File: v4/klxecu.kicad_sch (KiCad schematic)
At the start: 15 parts, among them J1 cam_sensor, J2 Conn_01x06, U1 S36B-WPZK-A, U2 LM2940S-5.0/NOPB, U3 Arduino Mega 2560 Pro

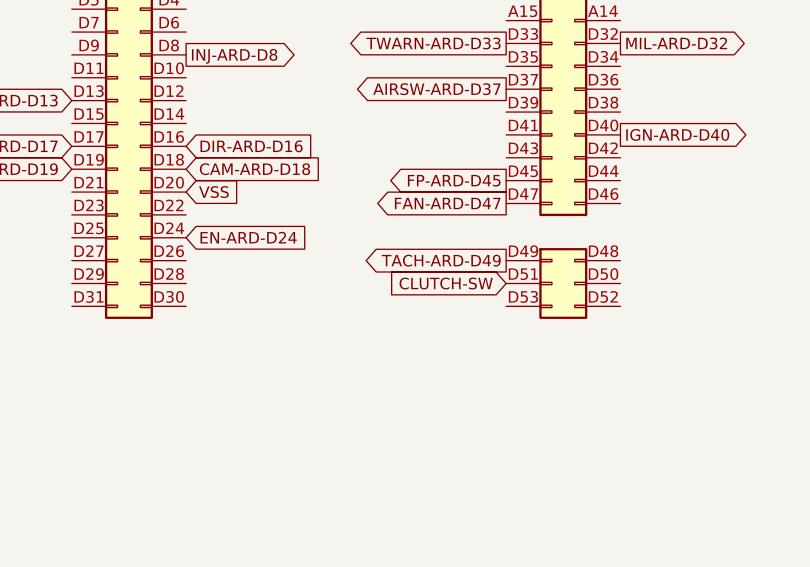
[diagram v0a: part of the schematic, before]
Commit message: V4 potential design
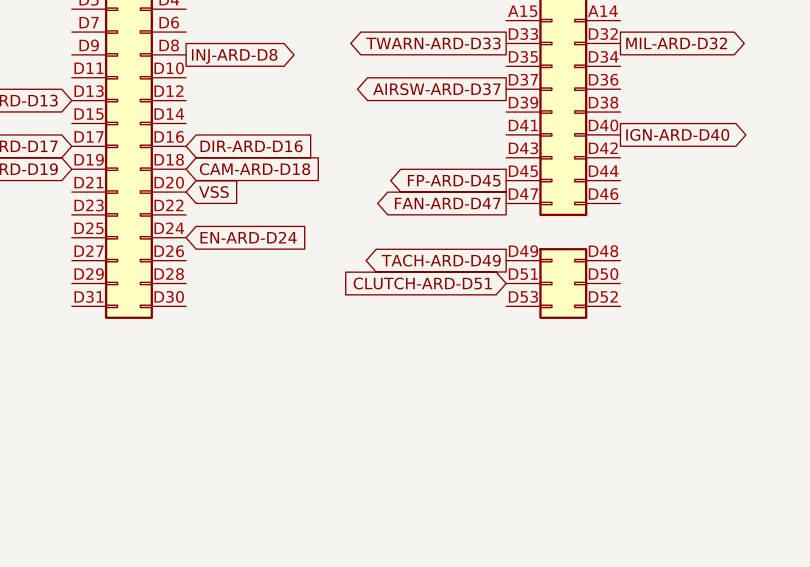
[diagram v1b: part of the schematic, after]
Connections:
- net CLUTCH-SW: no longer U3.D51
- new net CLUTCH-ARD-D51: U3.D51
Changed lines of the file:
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@@
     )
   )
-  (global_label "CLUTCH-SW" (shape input) (at 207.01 74.93 180) (fields_autoplaced)
+  (global_label "CLUTCH-ARD-D51" (shape input) (at 207.01 74.93 180) (fields_autoplaced)
     (effects (font (size 1.27 1.27)) (justify right))
-    (property "Intersheet References" "${INTERSHEET_REFS}" (id 0) (at 193.1669 75.0094 0)
+    (property "Intersheet References" "${INTERSHEET_REFS}" (id 0) (at 186.9379 74.8506 0)
       (effects (font (size 1.27 1.27)) (justify right) hide)
     )
@@
       (reference "#PWR015") (unit 1) (value "GND") (footprint "")
     )
+    (path "/98f72596-e058-4dba-8464-025a303cdc65/3d86f0fa-0e60-4863-ba29-c0c85017bc4d"
+      (reference "#PWR016") (unit 1) (value "GND") (footprint "")
+    )
     (path "/98f72596-e058-4dba-8464-025a303cdc65/08853ee7-ee30-4eb8-9fd5-85f877d2780a"
       (reference "#PWR017") (unit 1) (value "+5V") (footprint "")
@@
       (reference "J5") (unit 1) (value "IGN_ARD_OUT") (footprint "Connector_PinHeader_2.54mm:PinHeader_1x01_P2.54mm_Vertical")
     )
+    (path "/98f72596-e058-4dba-8464-025a303cdc65/4465d8d6-44cc-4706-b07c-4a5a0e286548"
+      (reference "J6") (unit 1) (value "Conn_01x01_Male") (footprint "Connector_PinHeader_2.54mm:PinHeader_1x01_P2.54mm_Vertical")
+    )
     (path "/a01c941e-2669-451e-92d9-4d3556674fec/a7d69894-f3b3-4f69-9136-a30ba4c9b64a"
       (reference "J7") (unit 1) (value "IGN_CONN") (footprint "Connector_PinHeader_2.54mm:PinHeader_1x01_P2.54mm_Vertical")
@@
       (reference "J8") (unit 1) (value "TACH_OUT") (footprint "Connector_PinHeader_2.54mm:PinHeader_1x01_P2.54mm_Vertical")
     )
+    (path "/98f72596-e058-4dba-8464-025a303cdc65/9d64ddb8-4723-4c2f-918d-32a269efe966"
+      (reference "J9") (unit 1) (value "Conn_01x01_Male") (footprint "Connector_PinHeader_2.54mm:PinHeader_1x01_P2.54mm_Vertical")
+    )
     (path "/98f72596-e058-4dba-8464-025a303cdc65/5abfb4a7-b746-40aa-8779-e189eca29e83"
       (reference "JP1") (unit 1) (value "Jumper_3_Open") (footprint "Connector_PinHeader_2.54mm:PinHeader_1x03_P2.54mm_Vertical")
@@
       (reference "JP7") (unit 1) (value "Jumper_2_Open") (footprint "Connector_PinHeader_2.54mm:PinHeader_1x02_P2.54mm_Vertical")
     )
+    (path "/98f72596-e058-4dba-8464-025a303cdc65/70c043b9-58b8-4e28-aee8-53d456176d44"
+      (reference "JP8") (unit 1) (value "SolderJumper_2_Open") (footprint "Jumper:SolderJumper-2_P1.3mm_Open_RoundedPad1.0x1.5mm")
+    )
+    (path "/98f72596-e058-4dba-8464-025a303cdc65/17c587ec-f90e-496b-9d29-3e30ce25c481"
+      (reference "JP9") (unit 1) (value "SolderJumper_2_Open") (footprint "Jumper:SolderJumper-2_P1.3mm_Open_RoundedPad1.0x1.5mm")
+    )
+    (path "/98f72596-e058-4dba-8464-025a303cdc65/4f510b35-3382-44bb-98c3-ff1c10450230"
+      (reference "JP10") (unit 1) (value "SolderJumper_2_Open") (footprint "Jumper:SolderJumper-2_P1.3mm_Open_RoundedPad1.0x1.5mm")
+    )
+    (path "/98f72596-e058-4dba-8464-025a303cdc65/28f99b34-5e15-4cf2-95f5-4e3fcbfe49c3"
+      (reference "JP11") (unit 1) (value "SolderJumper_2_Open") (footprint "Jumper:SolderJumper-2_P1.3mm_Open_RoundedPad1.0x1.5mm")
+    )
+    (path "/98f72596-e058-4dba-8464-025a303cdc65/c32fb5a6-3f52-42b3-8a4b-cc2ffe7bf7ed"
+      (reference "JP12") (unit 1) (value "SolderJumper_2_Open") (footprint "Jumper:SolderJumper-2_P1.3mm_Open_RoundedPad1.0x1.5mm")
+    )
     (path "/a01c941e-2669-451e-92d9-4d3556674fec/a246c3a3-766a-4abe-89a4-b39b374a1baf"
       (reference "Q1") (unit 1) (value "SSM3K357R") (footprint "Package_TO_SOT_SMD:SOT-23")
@@
       (reference "R2") (unit 1) (value "1k") (footprint "Resistor_THT:R_Axial_DIN0204_L3.6mm_D1.6mm_P5.08mm_Horizontal")
     )
+    (path "/98f72596-e058-4dba-8464-025a303cdc65/d8cf82da-4d4e-4bdd-9551-33d82e96b26c"
+      (reference "R3") (unit 1) (value "470") (footprint "Resistor_THT:R_Axial_DIN0204_L3.6mm_D1.6mm_P5.08mm_Horizontal")
+    )
     (path "/98f72596-e058-4dba-8464-025a303cdc65/54e1237d-4fb9-43d8-b6da-d31b711bf20a"
       (reference "R4") (unit 1) (value "2.49K") (footprint "Resistor_THT:R_Axial_DIN0204_L3.6mm_D1.6mm_P5.08mm_Horizontal")
@@
       (reference "U4") (unit 1) (value "TC4424AVPA") (footprint "Package_DIP:DIP-8_W7.62mm_Socket")
     )
-  )
+    (path "/98f72596-e058-4dba-8464-025a303cdc65/0ad112f2-a740-44fb-85f3-8fb336794c0a"
+      (reference "U5") (unit 1) (value "74HC4050") (footprint "Package_DIP:DIP-16_W7.62mm_LongPads")
+    )
+    (path "/98f72596-e058-4dba-8464-025a303cdc65/5049c04f-e24d-4558-b516-d38f68217582"
+      (reference "U5") (unit 2) (value "74HC4050") (footprint "Package_DIP:DIP-16_W7.62mm_LongPads")
+    )
+    (path "/98f72596-e058-4dba-8464-025a303cdc65/13dbb716-4f44-409c-93fa-ed732aa8ba2d"
+      (reference "U5") (unit 3) (value "74HC4050") (footprint "Package_DIP:DIP-16_W7.62mm_LongPads")
+    )
+    (path "/98f72596-e058-4dba-8464-025a303cdc65/345bfe3c-a708-4296-a475-9a2b36672c35"
+      (reference "U5") (unit 4) (value "74HC4050") (footprint "Package_DIP:DIP-16_W7.62mm_LongPads")
+    )
+    (path "/98f72596-e058-4dba-8464-025a303cdc65/adf1b474-a5ed-4d7d-8bbd-7032617448ee"
+      (reference "U5") (unit 5) (value "74HC4050") (footprint "Package_DIP:DIP-16_W7.62mm_LongPads")
+    )
+    (path "/98f72596-e058-4dba-8464-025a303cdc65/a9cc6fdb-1409-4597-8f07-5e119b64fb95"
+      (reference "U5") (unit 6) (value "74HC4050") (footprint "Package_DIP:DIP-16_W7.62mm_LongPads")
+    )
+    (path "/98f72596-e058-4dba-8464-025a303cdc65/f649c06a-975c-4901-a854-2516dd837f8c"
+      (reference "U5") (unit 7) (value "74HC4050") (footprint "Package_DIP:DIP-16_W7.62mm_LongPads")
+    )
+  )
